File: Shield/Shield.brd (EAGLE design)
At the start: 174 x 56 mm, 15 parts

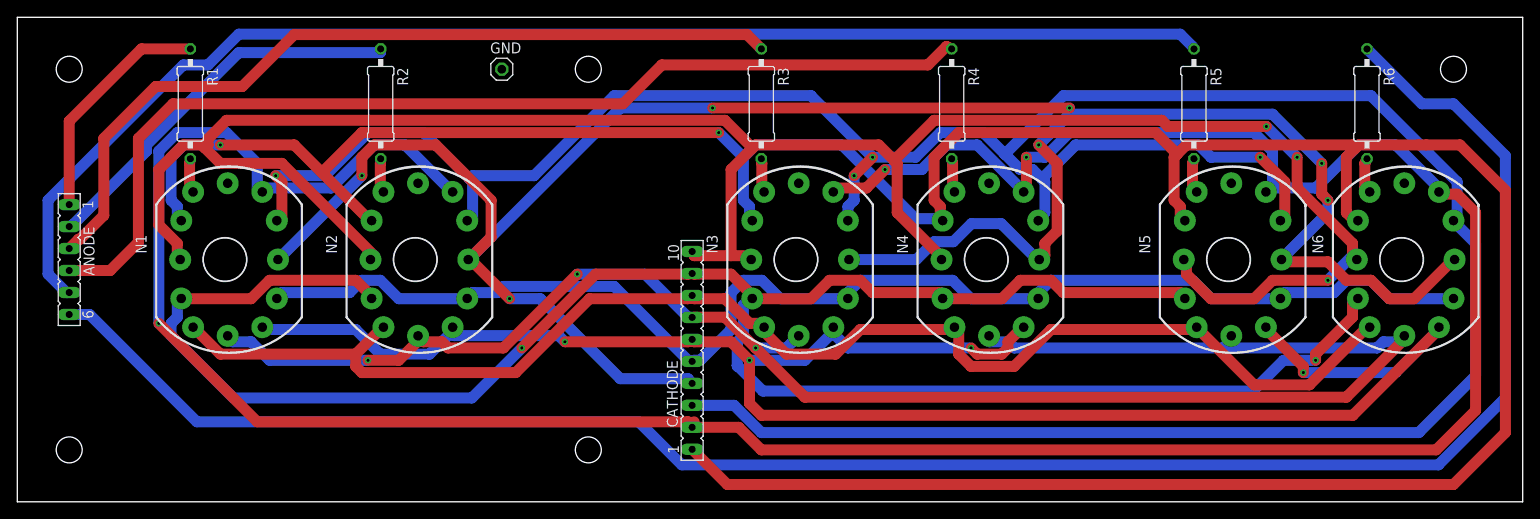
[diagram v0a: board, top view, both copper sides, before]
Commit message: forgot to save before commit... Comment: See last commit
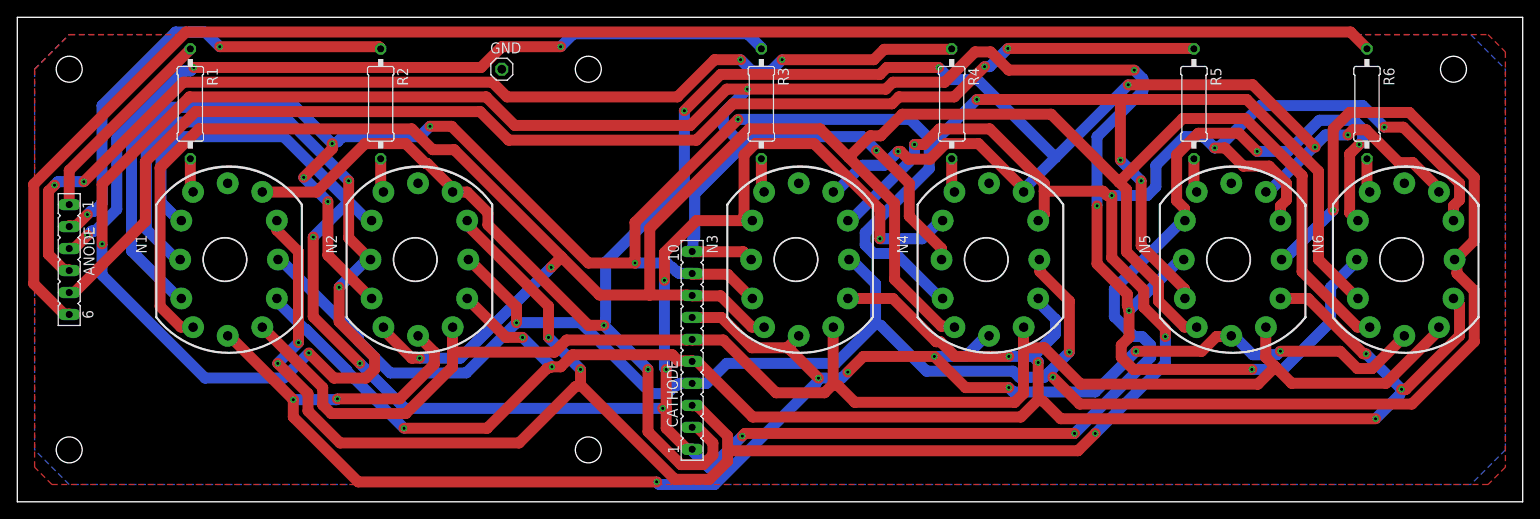
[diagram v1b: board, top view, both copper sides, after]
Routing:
- net 9: track 251.5 -> 392.1 mm, vias 3 -> 10
- net 7: track 162.7 -> 298.3 mm, vias 0 -> 2
- net 1: track 344.1 -> 253.7 mm, vias 3 -> 8
- net 4: track 155.2 -> 229.5 mm, vias 0 -> 8
- net 0: track 345.2 -> 299.0 mm, vias 2 -> 10
- net N$2: track 225.5 -> 179.3 mm
- net 8: track 247.8 -> 291.8 mm, vias 2 -> 9
- net 2: track 342.0 -> 306.3 mm, vias 4 -> 10
- net 5: track 213.3 -> 178.5 mm, vias 4 -> 0
- net 3: track 265.5 -> 253.2 mm, vias 7 -> 4
- net N$4: track 45.1 -> 52.8 mm, vias 0 -> 2
- net N$3: track 153.0 -> 148.5 mm, vias 0 -> 2
- net N$6: track 119.8 -> 124.2 mm, vias 0 -> 4
- net N$1: track 27.1 -> 23.8 mm
- net 6: track 208.6 -> 207.3 mm, vias 3 -> 9
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- added copper zone on layer 16, net GND
- added copper zone on layer 1, net N$8
